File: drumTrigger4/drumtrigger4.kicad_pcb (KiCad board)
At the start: 2 copper layers, 23 parts, among them J1 Input, J2 TrigOut, J3 CVout, J4 Power, U1 TL074

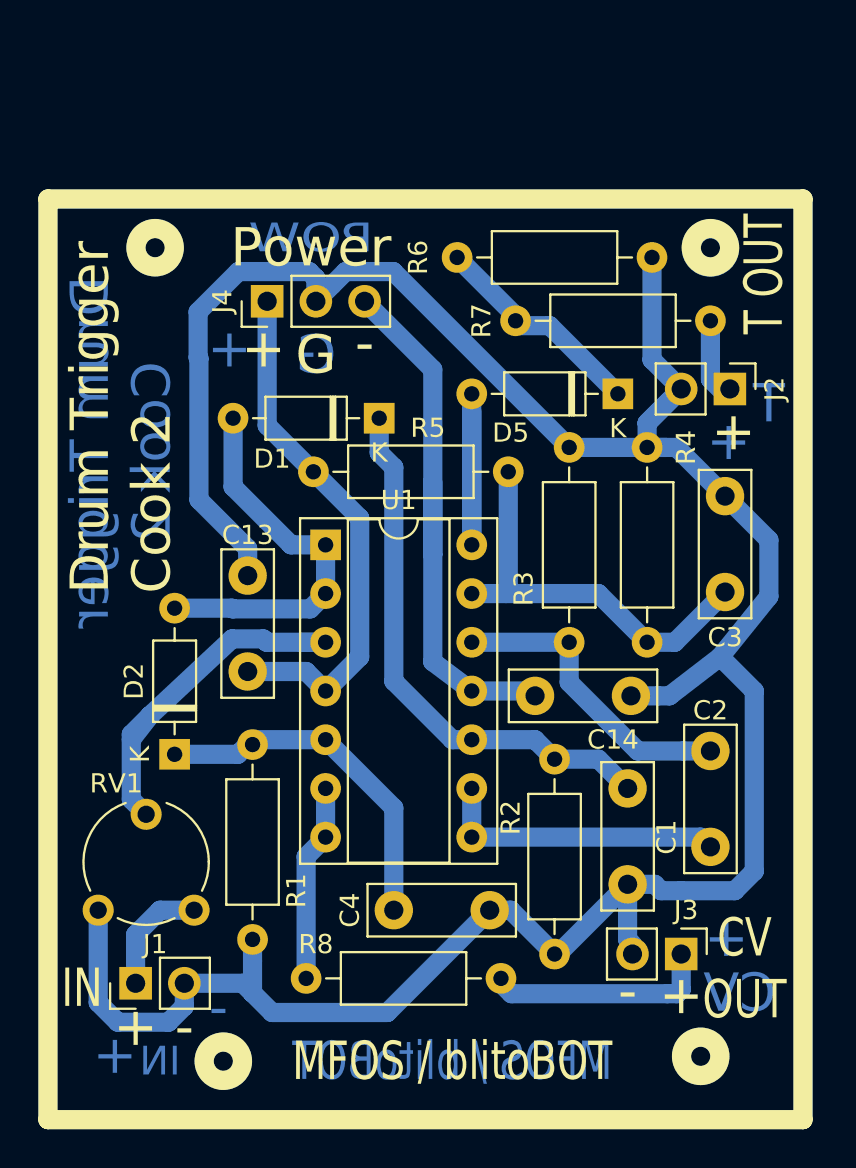
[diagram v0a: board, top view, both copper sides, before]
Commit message: experimenting with adding input gain, likely swap input pot next
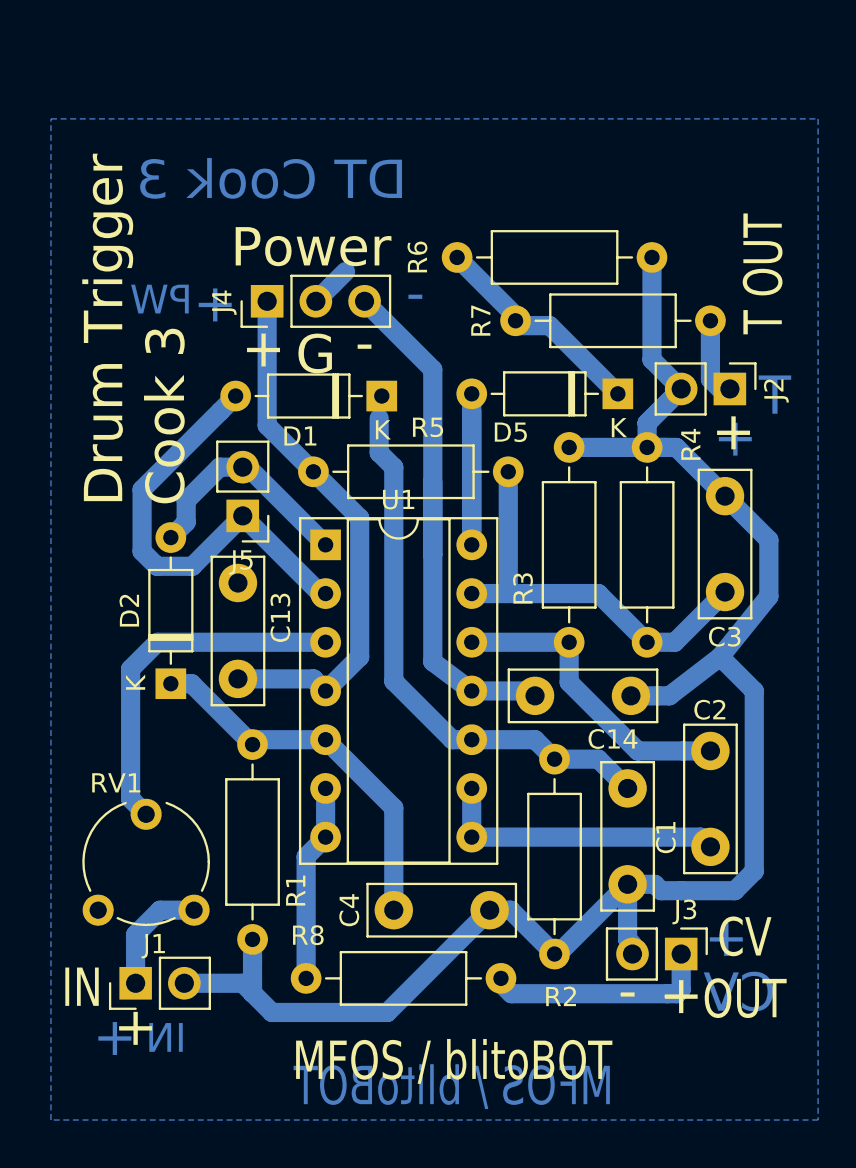
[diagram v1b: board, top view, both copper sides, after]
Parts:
- added J5: Gain, Connector_PinHeader_2.54mm:PinHeader_1x02_P2.54mm_Vertical, F.Cu at (143.0, 78.5)
- moved D2 3.69 mm to (139.2, 87.2)
- moved D1 1.16 mm to (150.2, 72.2)
- moved C13 0.64 mm to (142.8, 87.0)
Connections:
- D2 pad 2: Net-(D1-Pad2) -> Net-(D2-Pad2)
- U1 pad 1: Net-(D1-Pad2) -> Net-(D2-Pad2)
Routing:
- net GND: track 144.8 -> 94.9 mm
- net Net-(D2-Pad2): track 0.00 -> 11.9 mm
- net Net-(D1-Pad2): track 20.4 -> 22.8 mm
- net Net-(C4-Pad1): track 18.6 -> 19.7 mm
- net Net-(RV1-Pad2): track 19.6 -> 18.7 mm
- added copper zone on B.Cu, net GND
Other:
- board text added: "DT Cook 3"
- board text added: "Drum Trigger Cook 3"
- board text added: "PW"
- board text removed: "Drum Trigger Cook 2"
- board text removed: "POW"
